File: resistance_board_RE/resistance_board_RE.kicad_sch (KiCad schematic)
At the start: 178 parts, among them J1 Red Wire, J2 Blrown Wire, J3 Yellow Wire, J4 Black Wire, J5 Green Wire, J6 Orange Wire, M103 LTC1052CSW-PBF, M104 MC33071, M203 LTC1052CSW-PBF, Q1 FZT658, Q10 MMBF5485 "6M", Q104 SST404, Q11 MMBF5485 "6M", Q12 BC856 "3DW", Q13 FZT493, Q14 TIP32CG Heatsunk, Q15 FZT658, Q16 BC856 "3DW", Q17 BC846 "1DW", Q18 BC846 "1DW", Q19 BC846 "1DW", Q2 TIP32CG Heatsunk, Q20 BC846 "1DW", Q21 FZT758, Q22 BC846 "1DW", Q23 BC856 "3DW", Q24 BC846 "1DW", Q3 04N80C3, Q4 FZT758, Q5 TIP32CG Heatsunk, Q6 Q_PMOS_GDS, Q7 BC856 "3DW", Q8 TIP31AG Heatsunk, Q9 BC846 "1DW", U1 PVI5080N, U10 TL071, U2 LM337_TO220, U3 PVI5080N, U4 LTC1150, U5 DG211, U6 TL071, U7 LTC1150, U8 LTC1150, U9 TL071

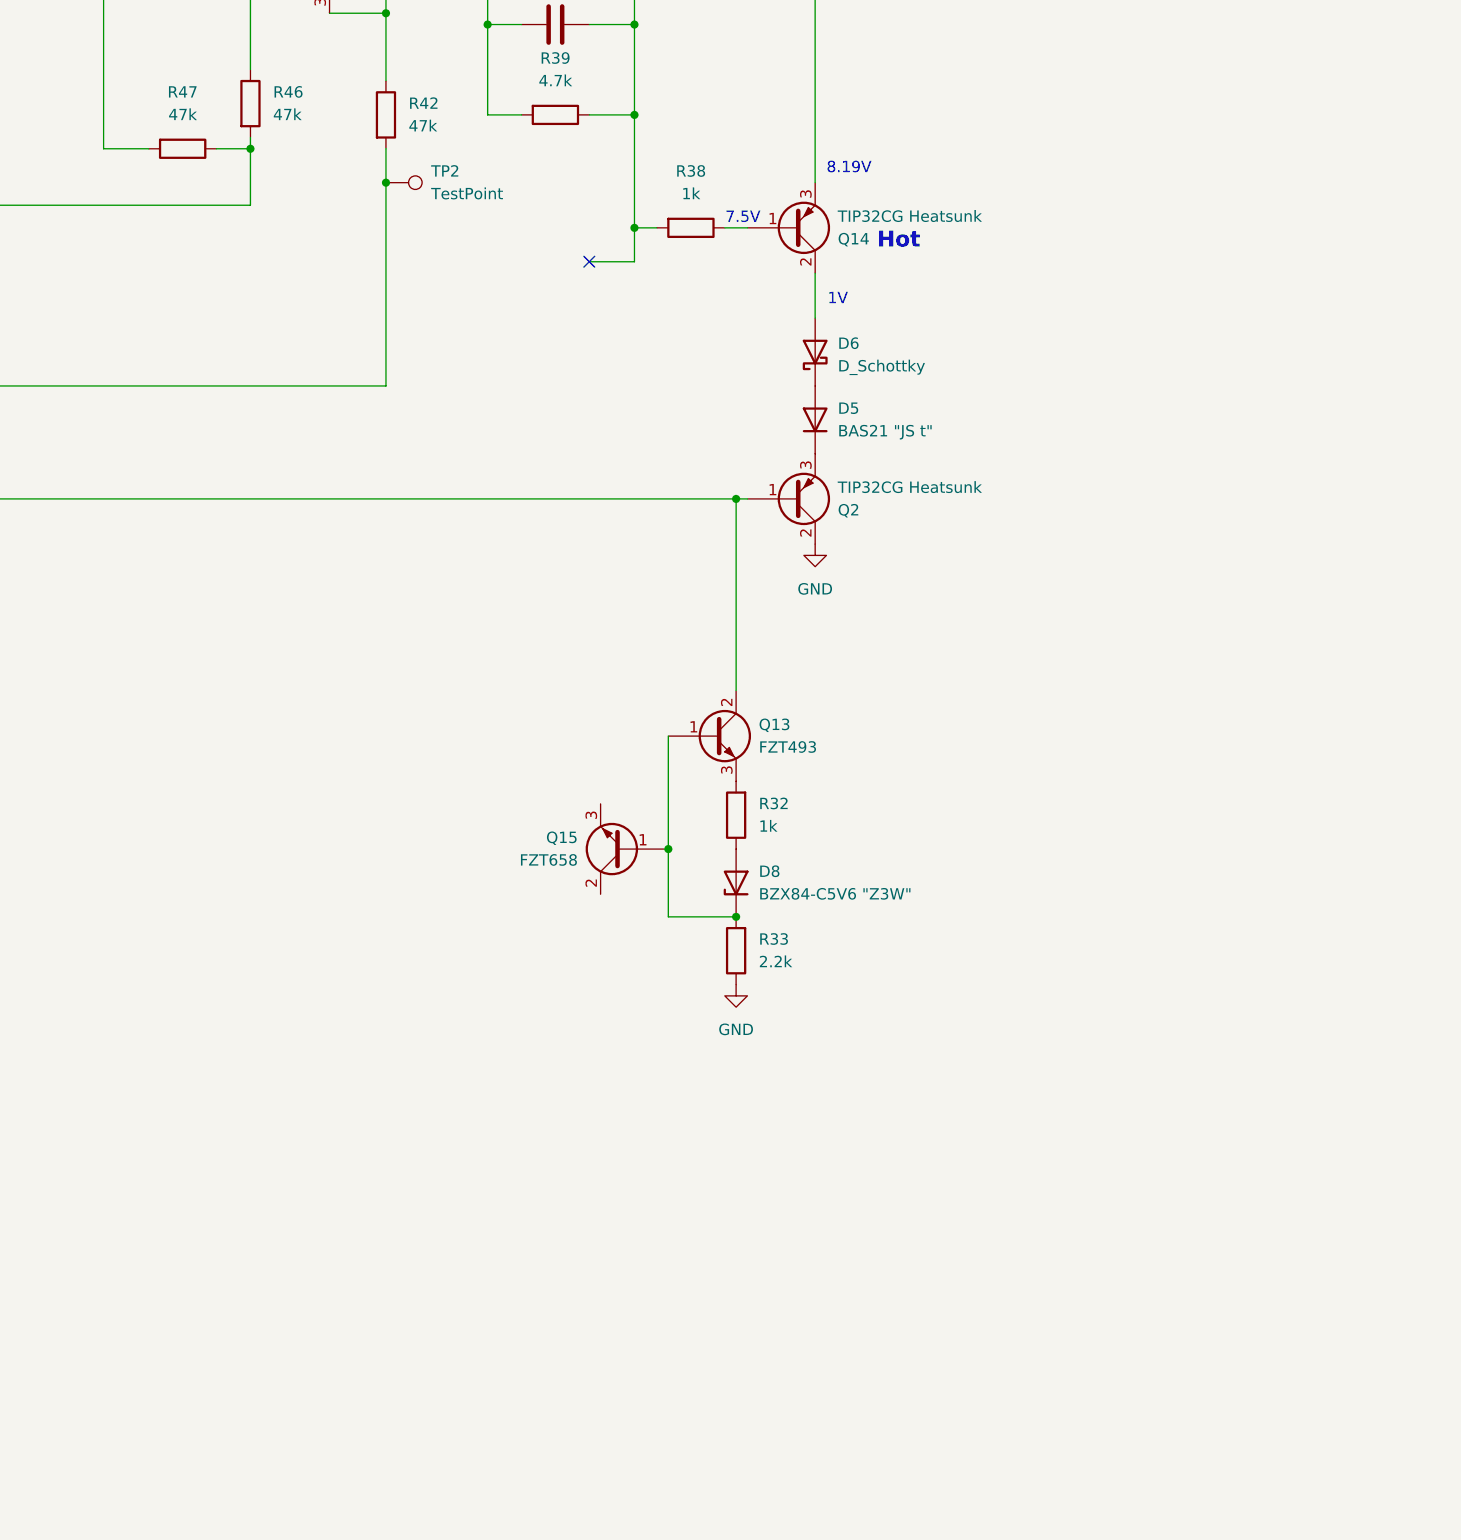
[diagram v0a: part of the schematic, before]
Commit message: asdf
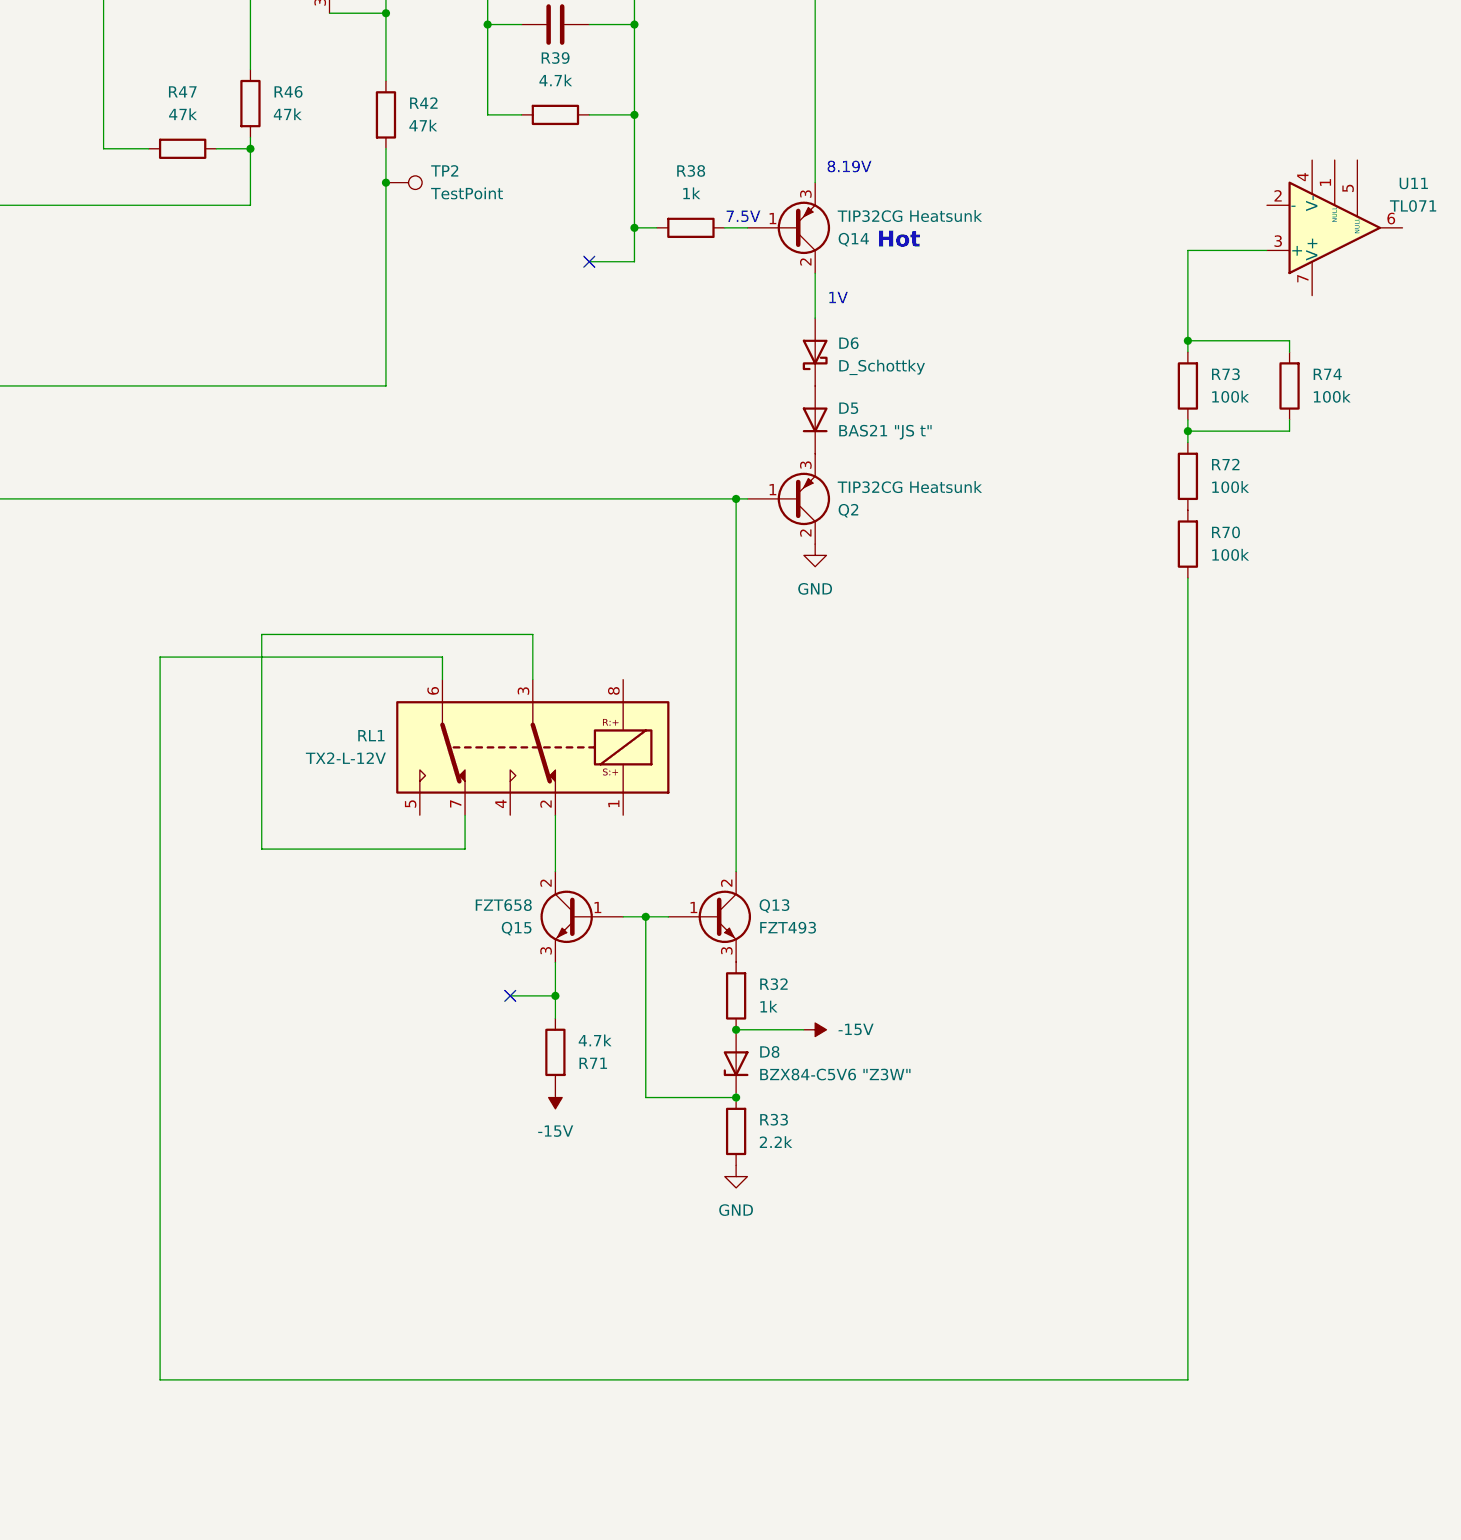
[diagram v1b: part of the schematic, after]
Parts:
- added R70, R72, R73, R74: 100k, symbol Device:R
- added R71: 4.7k, symbol Device:R
- added RL1: TX2-L-12V, symbol Relay:G6KU-2
- added U11: TL071, symbol Amplifier_Operational:TL071
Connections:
- net -15V: now reaches D8.1 (A), R32.1
- net -15V: now also R71.2
- net at Q15.2 (C): now also RL1.2
- net at Q15.3 (E): now also R71.1
- new net: RL1.3, RL1.7
- new net: R70.1, RL1.6
- new net: R70.2, R72.1
- new net: R72.2, R73.1, R74.1
- new net: R73.2, R74.2, U11.3 (+)
- no-connect marks 4 -> 5
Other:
- moved on the sheet: D8, Q13, Q15, R32, R33
